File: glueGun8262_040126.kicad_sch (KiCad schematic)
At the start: 75 parts, among them CN1 KF243-5.0-2P, CN2 KF243-5.0-2P, CN3 KF243-5.0-2P, CN4 KF243-5.0-2P, CN5 KF243-5.0-2P, CN6 KF243-5.0-2P, CN7 KF243-5.0-2P, CN9 KF243-5.0-4P, Q1 SQM120P10-10m1L, U1 DRV8262DDWR, U10 INA240A2DR, U11 INA240A2DR, U2 DRV8262DDWR, U3 ESP32-S3-DEVKITC-1-N8R8, U5 6N137, U6 INA240A2DR, U7 INA240A2DR, U8 K7805-1000R3_C2992391, U9 TLP291-4(V4GBTPE)

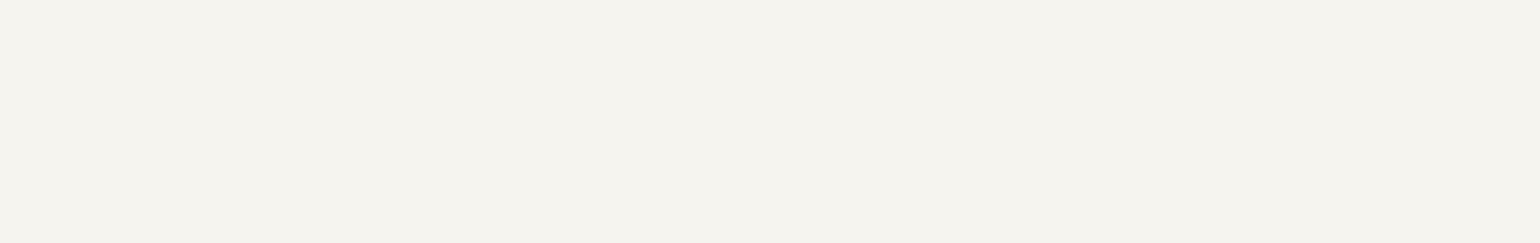
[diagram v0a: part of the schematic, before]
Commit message: before adding headers
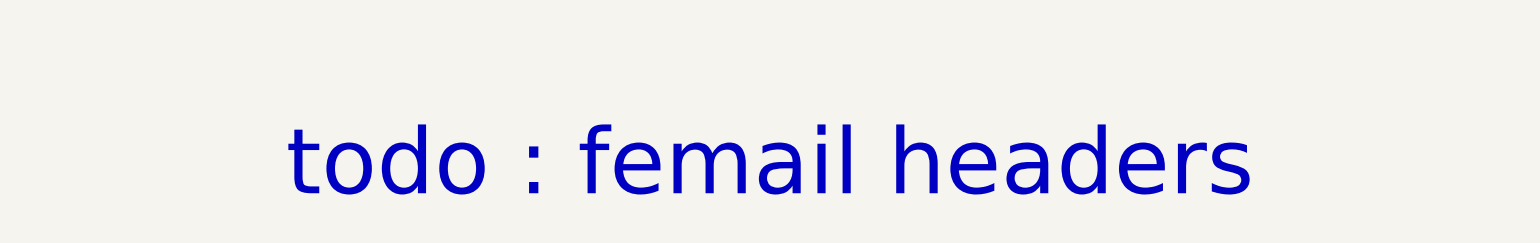
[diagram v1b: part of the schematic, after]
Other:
- note added: "todo : femail headers"
